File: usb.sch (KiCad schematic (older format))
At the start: 16 parts, among them J3 JTAG, U1 LFE5U-85F-6BG381C, Y1 FNETHE025

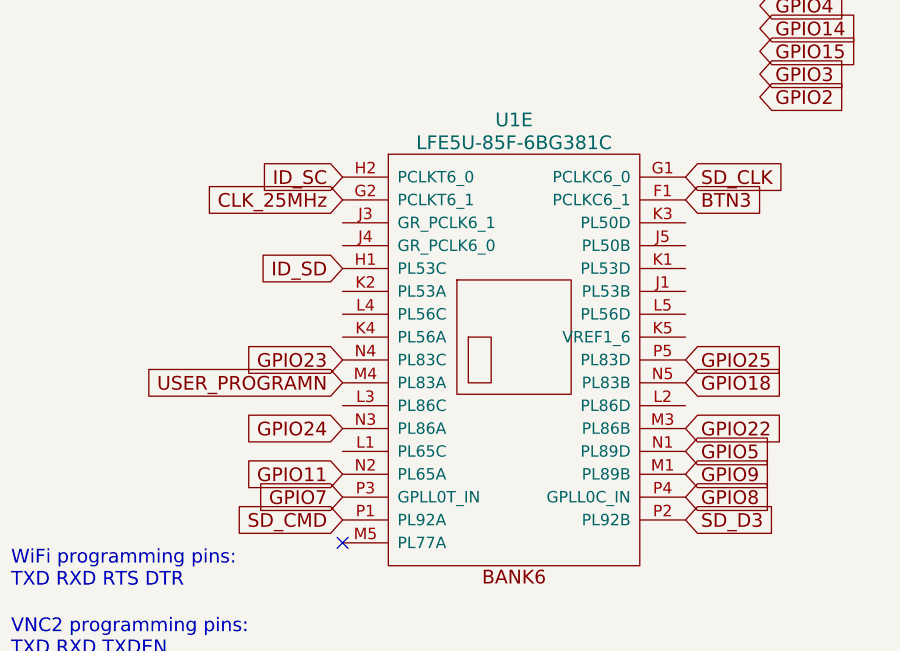
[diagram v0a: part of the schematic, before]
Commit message: Initial complete routing done
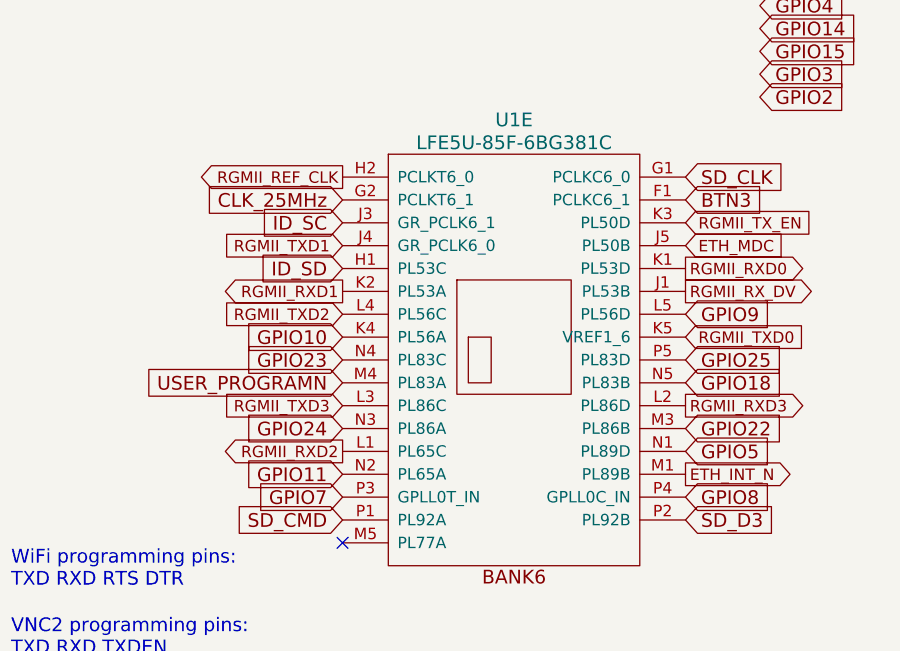
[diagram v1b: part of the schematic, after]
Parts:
- J3: footprint Connector_PinSocket_2.54mm:PinSocket_2x03_P2.54mm_Vertical -> Connector_PinHeader_1.00mm:PinHeader_2x03_P1.00mm_Vertical_SMD
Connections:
- net labels added: ETH_INT_N, ETH_MDC, GPIO10, RGMII_REF_CLK, RGMII_RXD0, RGMII_RXD1, RGMII_RXD2, RGMII_RXD3, RGMII_RX_DV, RGMII_TXD0, RGMII_TXD1, RGMII_TXD2, RGMII_TXD3, RGMII_TX_EN
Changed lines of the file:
@@
 $Descr A4 11693 8268
 encoding utf-8
-Sheet 6 12
+Sheet 6 13
 Title "ULX3S"
 Date ""
@@
 F 0 "J3" H 7300 5717 50  0000 C CNN
 F 1 "JTAG" H 7300 5626 50  0000 C CNN
-F 2 "Connector_PinSocket_2.54mm:PinSocket_2x03_P2.54mm_Vertical" H 7250 5400 50  0001 C CNN
+F 2 "Connector_PinHeader_1.00mm:PinHeader_2x03_P1.00mm_Vertical_SMD" H 7250 5400 50  0001 C CNN
 F 3 "~" H 7250 5400 50  0001 C CNN
 	1    7250 5400
@@
 Wire Wire Line
 	975  2225 1075 2225
-Text GLabel 10150 2650 2    60   Input ~ 0
+Text GLabel 10150 1950 2    60   Input ~ 0
 GPIO9
 Text GLabel 10150 1450 2    60   Input ~ 0
@@
 Text GLabel 8650 1750 0    60   Input ~ 0
 ID_SD
-Text GLabel 8650 1350 0    60   Input ~ 0
+Text GLabel 8650 1550 0    60   Input ~ 0
 ID_SC
-Text GLabel 10150 2550 2    60   Input ~ 0
-GPIO5
 Text GLabel 8650 2650 0    60   Input ~ 0
 GPIO11
 Text GLabel 10150 2450 2    60   Input ~ 0
 GPIO22
+Text GLabel 10150 1650 2    50   Input ~ 0
+ETH_MDC
+Text GLabel 10150 1850 2    50   Output ~ 0
+RGMII_RX_DV
+Text GLabel 8650 1350 0    50   Output ~ 0
+RGMII_REF_CLK
+Text GLabel 10150 2650 2    50   Output ~ 0
+ETH_INT_N
+Text GLabel 8650 2550 0    50   Output ~ 0
+RGMII_RXD2
+Text GLabel 8650 1850 0    50   Output ~ 0
+RGMII_RXD1
+Text GLabel 10150 1750 2    50   Output ~ 0
+RGMII_RXD0
+Text GLabel 8650 2350 0    50   Input ~ 0
+RGMII_TXD3
+Text GLabel 8650 1950 0    50   Input ~ 0
+RGMII_TXD2
+Text GLabel 8650 1650 0    50   Input ~ 0
+RGMII_TXD1
+Text GLabel 10150 2050 2    50   Input ~ 0
+RGMII_TXD0
+Text GLabel 10150 2550 2    60   Input ~ 0
+GPIO5
+Text GLabel 10150 1550 2    50   Input ~ 0
+RGMII_TX_EN
+Text GLabel 10150 2350 2    50   Output ~ 0
+RGMII_RXD3
+Text GLabel 8650 2050 0    60   Input ~ 0
+GPIO10
 $EndSCHEMATC
